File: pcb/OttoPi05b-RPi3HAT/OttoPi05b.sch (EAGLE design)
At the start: 26 parts

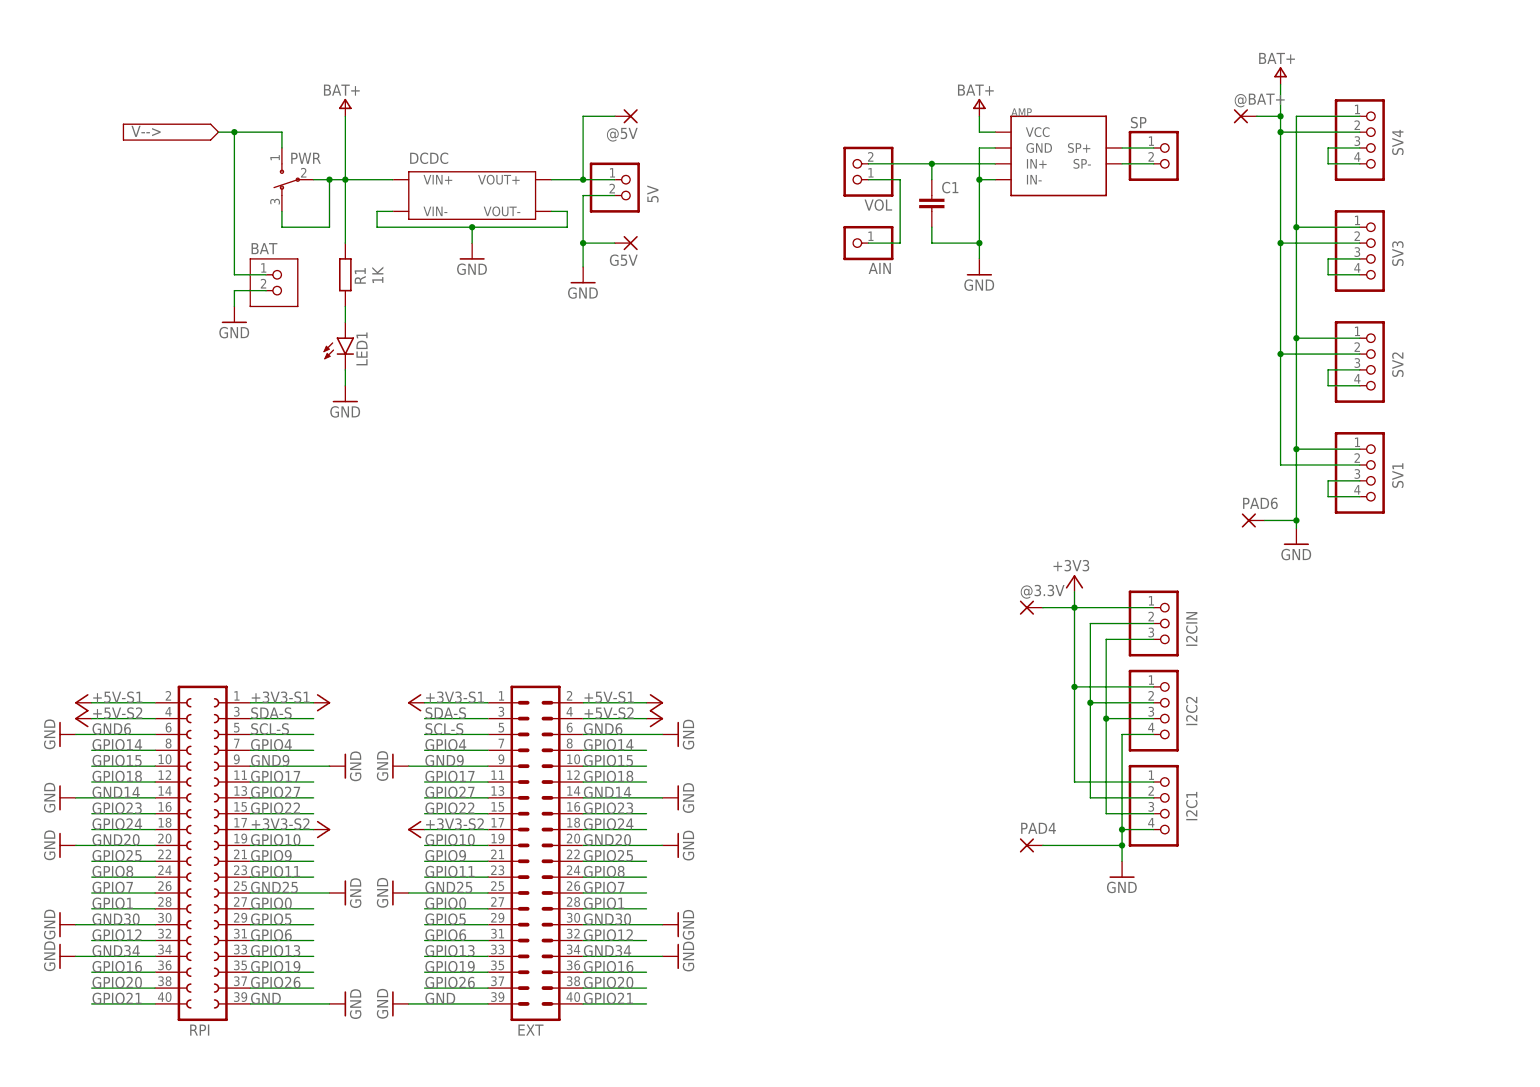
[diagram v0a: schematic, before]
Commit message: update
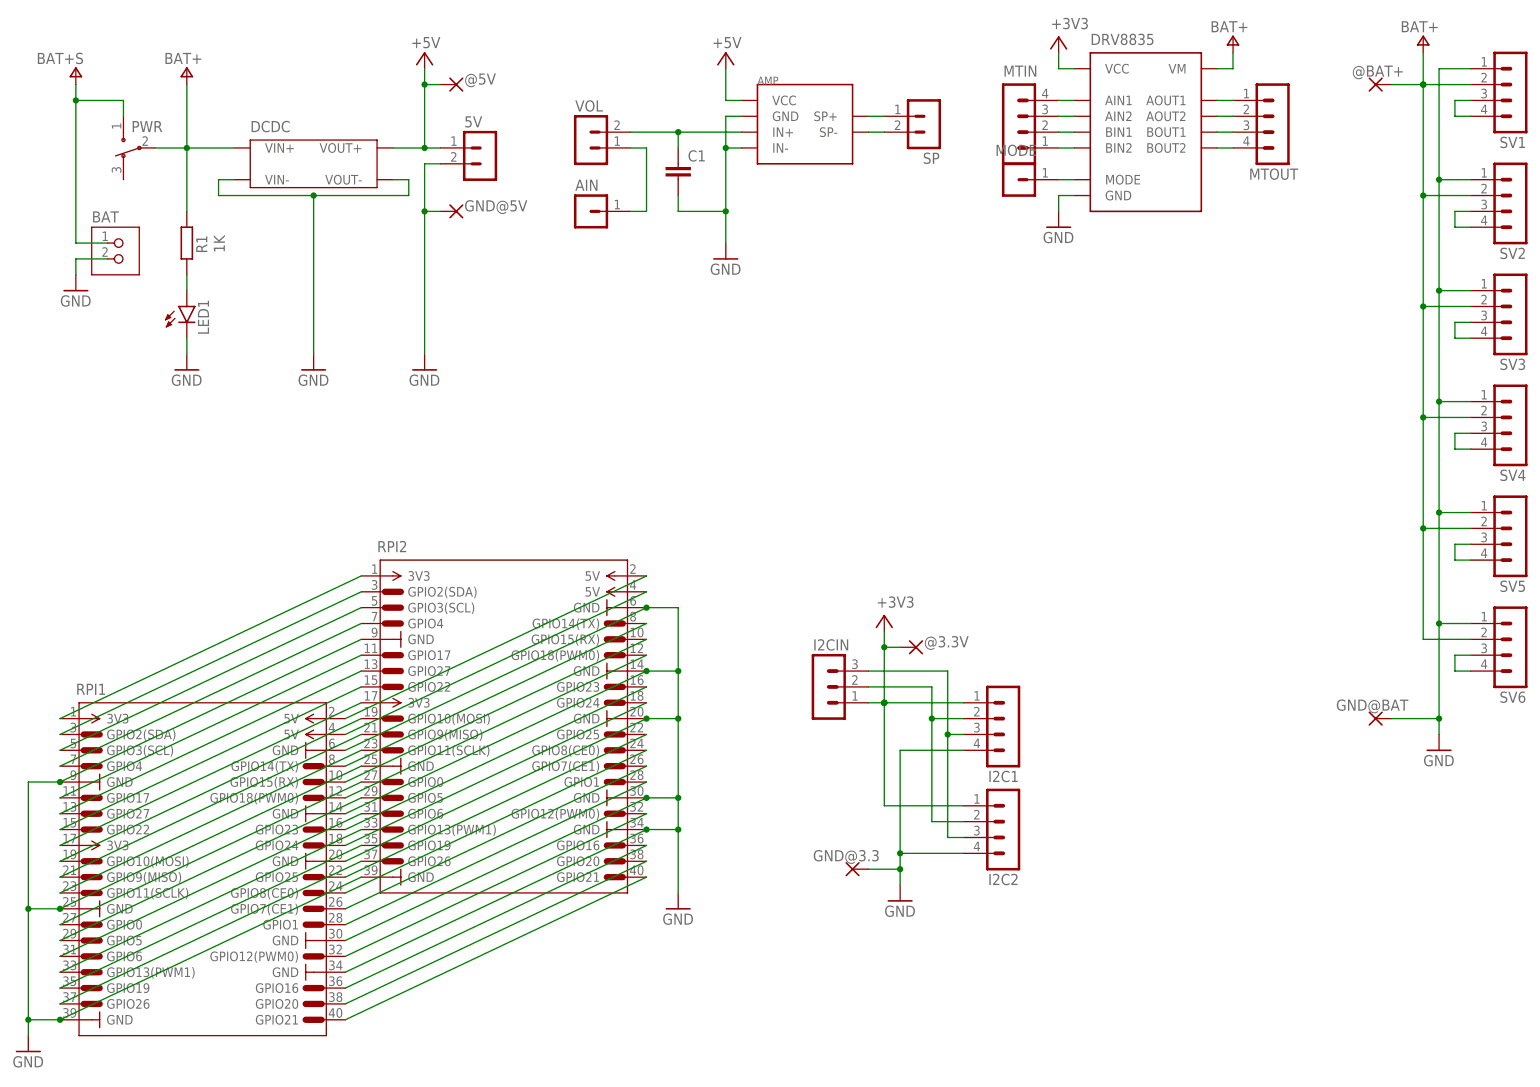
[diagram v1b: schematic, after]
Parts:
- removed EXT: (no value), con-lstb:MA20-2W
- removed G5V, PAD4, PAD6: (no value), wirepad:2,15/1,0
- removed RPI: (no value), con-lsta:FE20-2
- added DRV8835: (no value), ytani1:DRV8835MOD
- added GND@3.3, GND@5V, GND@BAT: (no value), wirepad:2,15/1,0
- added MODE: (no value), ytani-con-lstb:MA01-1
- added MTIN, MTOUT, SV5, SV6: (no value), ytani-con-lstb:MA04-1
- added RPI1, RPI2: (no value), ytani1:RPI-PIN
- 5V, SP, VOL: device pinhead:PINHD-1X2 -> ytani-con-lstb:MA02-1
- AIN: device pinhead:PINHD-1X1 -> ytani-con-lstb:MA01-1
- I2C1, I2C2, SV1, SV2, SV3, SV4: device pinhead:PINHD-1X4 -> ytani-con-lstb:MA04-1
- I2CIN: device pinhead:PINHD-1X3 -> ytani-con-lstb:MA03-1
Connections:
- net SV1 renamed N$1
- net SV2 renamed N$3
- net SV3 renamed N$4
- net SV4 renamed N$5
- removed net +3V3-S1: EXT.1, RPI.1
- removed net +3V3-S2: EXT.17, RPI.17
- removed net +5V-S1: EXT.2, RPI.2
- removed net +5V-S2: EXT.4, RPI.4
- removed net BAT+S: BAT.1, PWR.1
- removed net GND14: EXT.14, RPI.14
- removed net GND20: EXT.20, RPI.20
- removed net GND25: EXT.25, RPI.25
- removed net GND30: EXT.30, RPI.30
- removed net GND34: EXT.34, RPI.34
- removed net GND6: EXT.6, RPI.6
- removed net GND9: EXT.9, RPI.9
- removed net GPIO0: EXT.27, RPI.27
- removed net GPIO1: EXT.28, RPI.28
- removed net GPIO10: EXT.19, RPI.19
- removed net GPIO11: EXT.23, RPI.23
- removed net GPIO12: EXT.32, RPI.32
- removed net GPIO13: EXT.33, RPI.33
- removed net GPIO14: EXT.8, RPI.8
- removed net GPIO15: EXT.10, RPI.10
- removed net GPIO16: EXT.36, RPI.36
- removed net GPIO17: EXT.11, RPI.11
- removed net GPIO18: EXT.12, RPI.12
- removed net GPIO19: EXT.35, RPI.35
- removed net GPIO20: EXT.38, RPI.38
- removed net GPIO21: EXT.40, RPI.40
- removed net GPIO22: EXT.15, RPI.15
- removed net GPIO23: EXT.16, RPI.16
- removed net GPIO24: EXT.18, RPI.18
- removed net GPIO25: EXT.22, RPI.22
- removed net GPIO26: EXT.37, RPI.37
- removed net GPIO27: EXT.13, RPI.13
- removed net GPIO4: EXT.7, RPI.7
- removed net GPIO5: EXT.29, RPI.29
- removed net GPIO6: EXT.31, RPI.31
- removed net GPIO7: EXT.26, RPI.26
- removed net GPIO8: EXT.24, RPI.24
- removed net GPIO9: EXT.21, RPI.21
- removed net SCL-S: EXT.5, RPI.5
- removed net SDA-S: EXT.3, RPI.3
- new net N$10: RPI1.GPIO12(PWM0), RPI2.GPIO12(PWM0)
- new net N$11: DRV8835.BIN2, MTIN.1
- new net N$12: RPI1.GPIO1, RPI2.GPIO1
- new net N$13: RPI1.GPIO7(CE1), RPI2.GPIO7(CE1)
- new net N$14: RPI1.GPIO8(CE0), RPI2.GPIO8(CE0)
- new net N$15: RPI1.GPIO25, RPI2.GPIO25
- new net N$16: RPI1.5V@1, RPI2.5V@1
- new net N$17: RPI1.5V@2, RPI2.5V@2
- new net N$18: DRV8835.BIN1, MTIN.2
- new net N$19: RPI1.GPIO14(TX), RPI2.GPIO14(TX)
- new net N$2: SV5.3, SV5.4
- new net N$20: RPI1.GPIO15(RX), RPI2.GPIO15(RX)
- new net N$21: RPI1.GPIO18(PWM0), RPI2.GPIO18(PWM0)
- new net N$22: RPI1.GPIO23, RPI2.GPIO23
- new net N$23: RPI1.GPIO24, RPI2.GPIO24
- new net N$24: DRV8835.AIN2, MTIN.3
- new net N$25: DRV8835.AIN1, MTIN.4
- new net N$26: RPI1.3V3@1, RPI2.3V3@1
- new net N$27: RPI1.GPIO2(SDA), RPI2.GPIO2(SDA)
- new net N$28: RPI1.GPIO3(SCL), RPI2.GPIO3(SCL)
- new net N$29: RPI1.GPIO4, RPI2.GPIO4
- new net N$30: DRV8835.AOUT1, MTOUT.1
- new net N$31: RPI1.GPIO17, RPI2.GPIO17
- new net N$32: RPI1.GPIO27, RPI2.GPIO27
- new net N$33: RPI1.GPIO22, RPI2.GPIO22
- new net N$34: RPI1.GPIO11(SCLK), RPI2.GPIO11(SCLK)
- new net N$35: RPI1.GPIO10(MOSI), RPI2.GPIO10(MOSI)
- new net N$36: RPI1.GPIO9(MISO), RPI2.GPIO9(MISO)
- new net N$37: RPI1.3V3@2, RPI2.3V3@2
- new net N$38: RPI1.GPIO0, RPI2.GPIO0
- new net N$39: RPI1.GPIO5, RPI2.GPIO5
- new net N$40: RPI1.GPIO6, RPI2.GPIO6
- new net N$41: RPI1.GPIO13(PWM1), RPI2.GPIO13(PWM1)
- new net N$42: RPI1.GPIO19, RPI2.GPIO19
- new net N$43: RPI1.GPIO26, RPI2.GPIO26
- new net N$44: DRV8835.AOUT2, MTOUT.2
- new net N$45: DRV8835.BOUT1, MTOUT.3
- new net N$46: DRV8835.BOUT2, MTOUT.4
- new net N$47: SV6.3, SV6.4
- new net N$6: RPI1.GPIO21, RPI2.GPIO21
- new net N$7: RPI1.GPIO20, RPI2.GPIO20
- new net N$8: RPI1.GPIO16, RPI2.GPIO16
- new net N$9: DRV8835.MODE, MODE.1
- net +3V3: now also DRV8835.VCC
- net +5V: now also AMP.VCC
- net BAT+: now also DRV8835.VM, SV5.2, SV6.2; no longer PWR.3
- net GND: now also DRV8835.GND, GND@3.3.P, GND@5V.P, GND@BAT.P, RPI1.GND@1, RPI1.GND@2, RPI1.GND@3, RPI1.GND@4, RPI1.GND@5, RPI1.GND@6, RPI1.GND@7, RPI1.GND@8, RPI2.GND@1, RPI2.GND@2, RPI2.GND@3, RPI2.GND@4, RPI2.GND@5, RPI2.GND@6, RPI2.GND@7, RPI2.GND@8, SV5.1, SV6.1; no longer EXT.39, G5V.P, PAD4.P, PAD6.P, RPI.39
- net V+: now also BAT.1, PWR.1; no longer AMP.VCC
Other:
- moved on the sheet: 5V, @3.3V, @5V, @BAT+, AIN, AMP, BAT, C1, DCDC, LED1, PWR, R1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
